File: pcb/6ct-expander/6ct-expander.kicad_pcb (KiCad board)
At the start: 2 copper layers, 88 x 30 mm, 57 parts, among them J1 SJ-3524-SMT-TR, J2 SJ-3524-SMT-TR, J3 SJ-3524-SMT-TR, J4 SJ-3524-SMT-TR, J5 SJ-3524-SMT-TR, J6 SJ-3524-SMT-TR, J7 Conn_02x05_Odd_Even

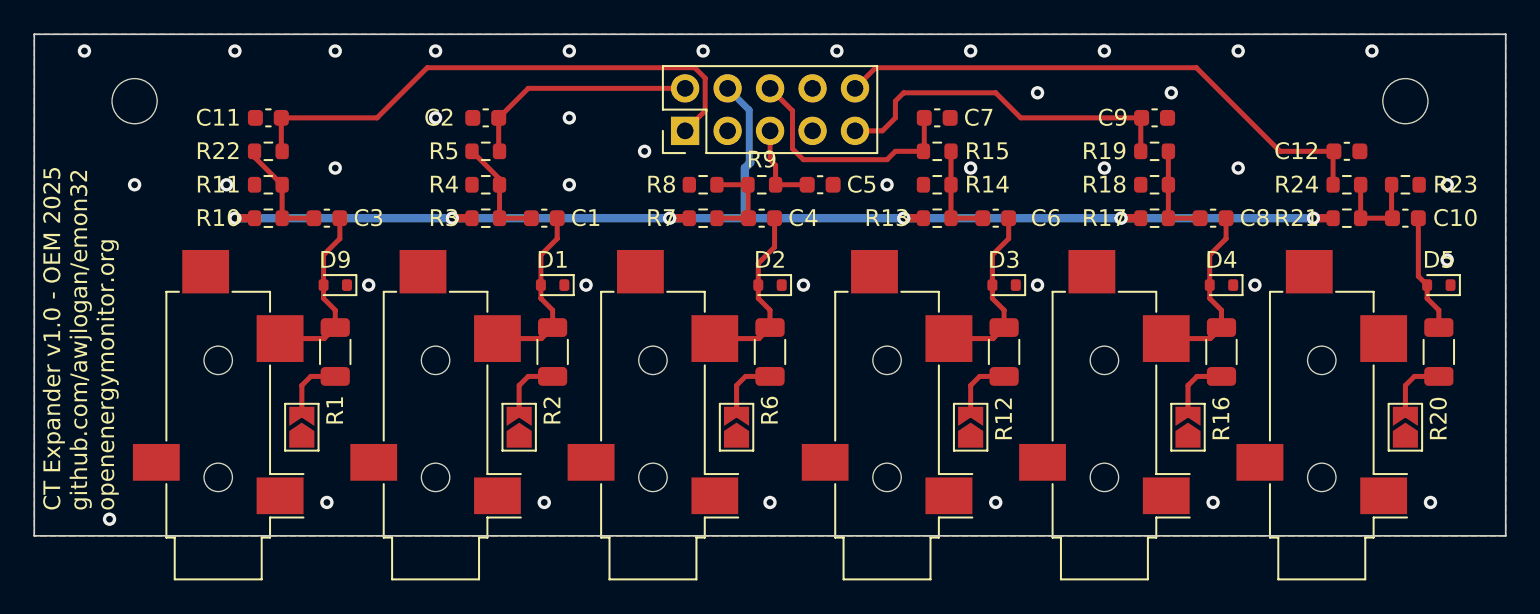
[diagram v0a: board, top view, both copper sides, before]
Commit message: Freeze for manufacture
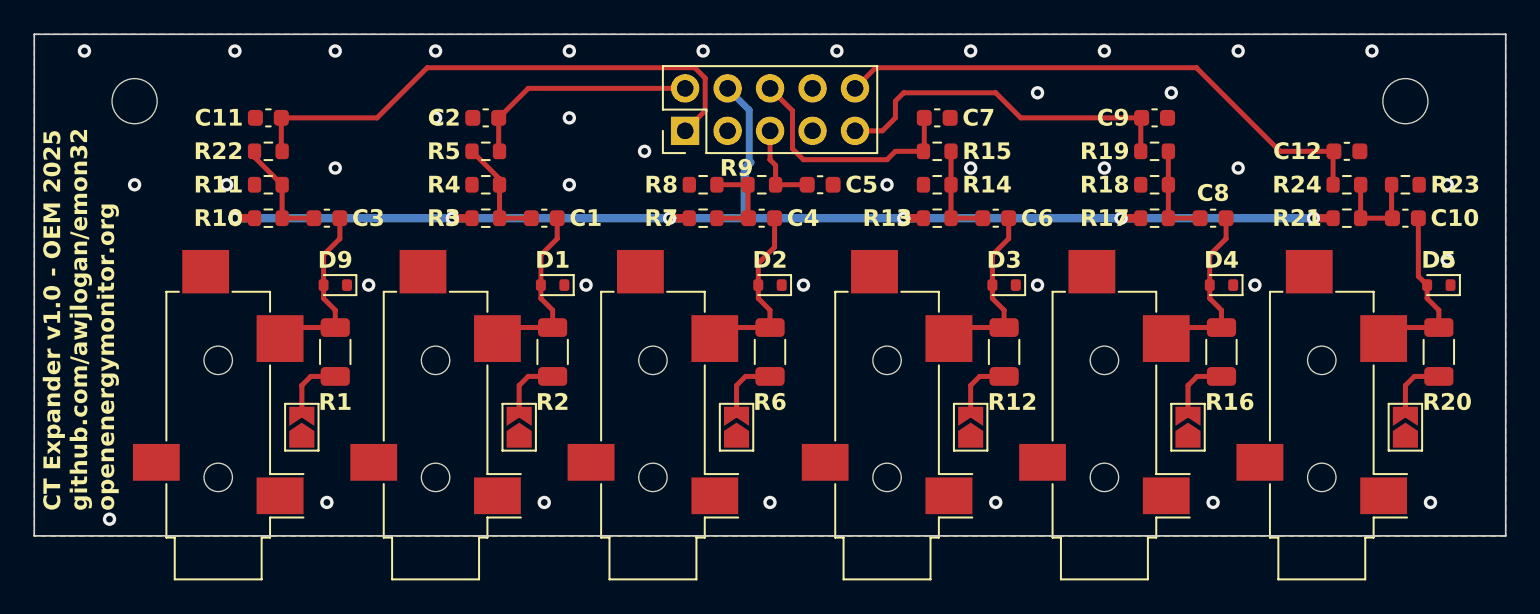
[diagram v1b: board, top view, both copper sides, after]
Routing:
- net Net-(D5-A2): track 7.04 -> 10.6 mm
